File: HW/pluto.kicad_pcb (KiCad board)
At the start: 4 copper layers, 99.8 x 99.8 mm, 68 parts, among them J1 VCC1, J10 GND3, J11 Expansion Bus, J12 VIA2PB, J2 GND1, J3 VCC2, J4 POWER, J5 GND2, J6 RS232a, J9 VCC3, P1 IDE0, Q1 DS1813, SW1 RESET, SW2 PANIC, U1 WD65C02PLCC44, U10 MAX232, U11 ST16C550PLCC44, U12 74LS03, U2 AT28HC256EPLCC32, U3 IS61C256AL-12JLI, U4 DS1511Y+, U5 TL7705B, U6 PlutoDecoder, U7 WD65C22PLCC44, U8 74HC74, U9 WD65C22PLCC44, X1 16MHz, X2 3.6864MHz

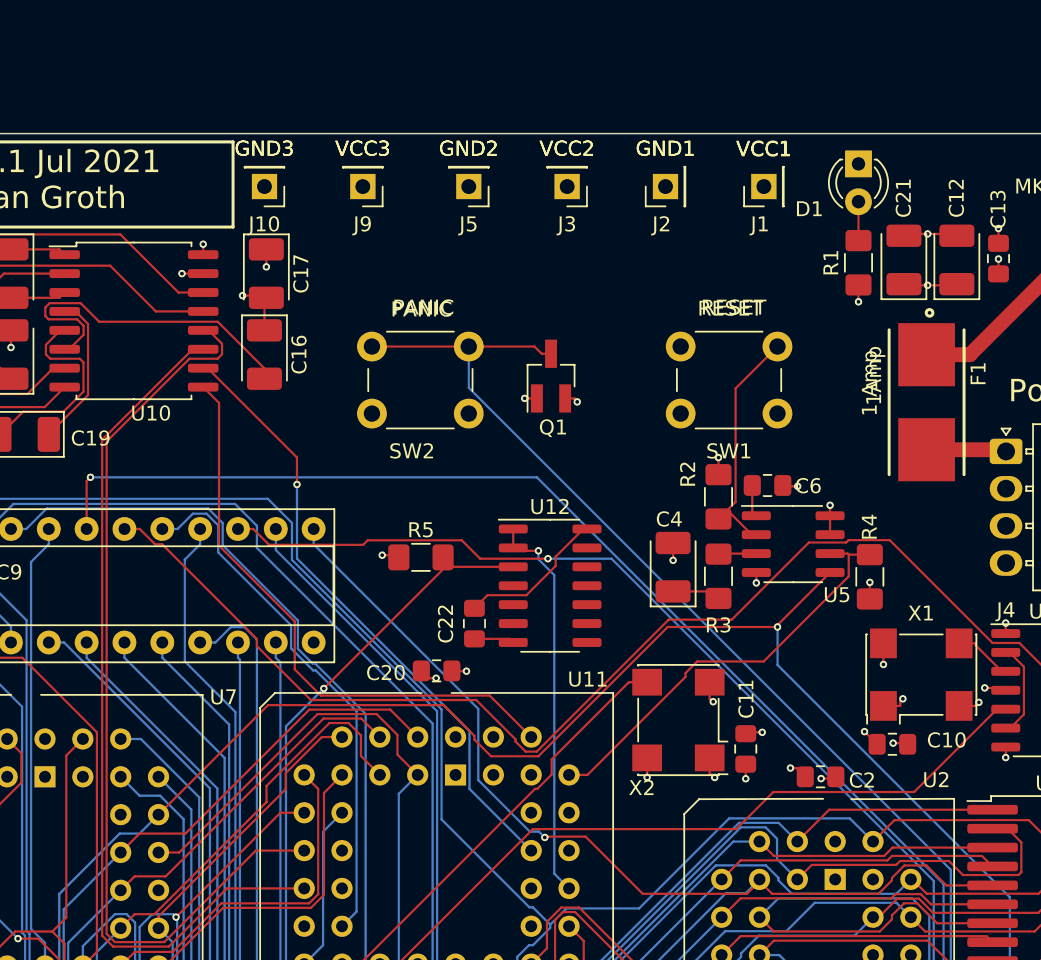
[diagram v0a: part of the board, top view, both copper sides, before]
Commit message: small updates
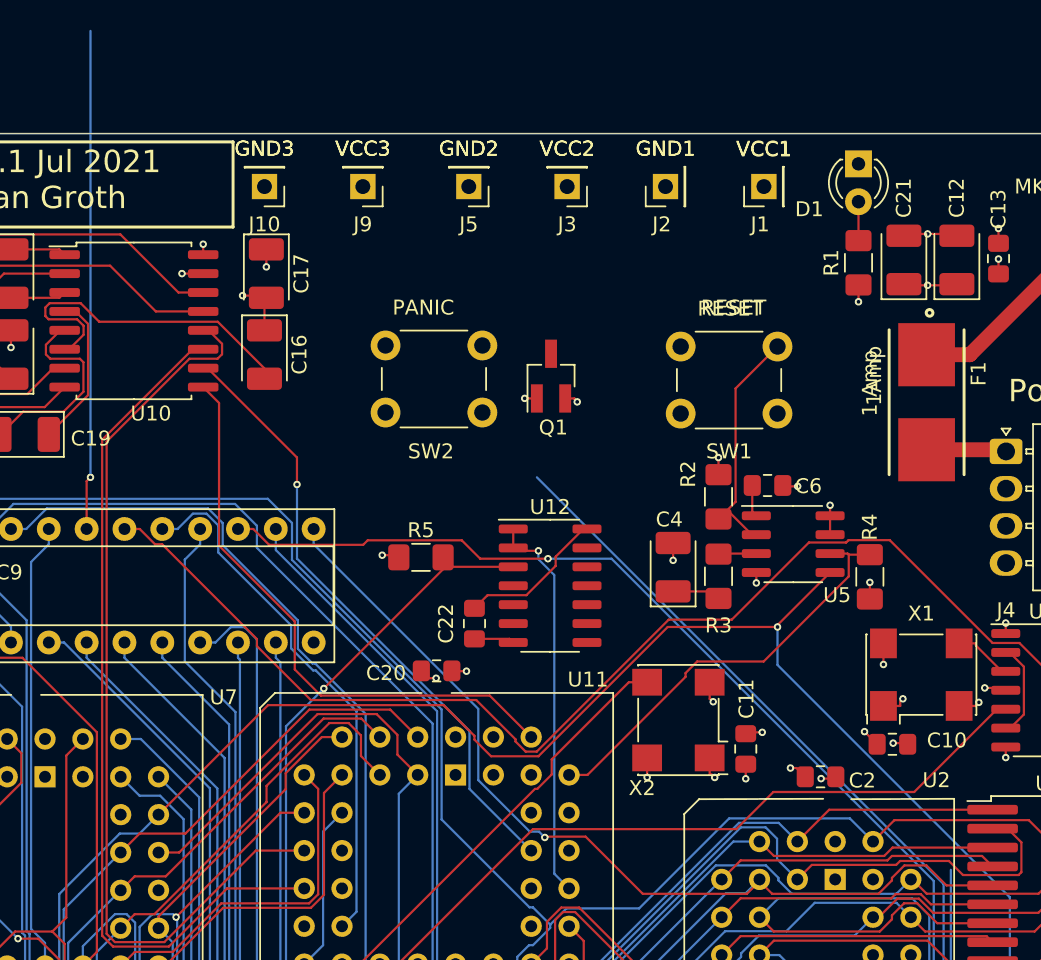
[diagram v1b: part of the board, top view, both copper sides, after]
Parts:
- moved SW2 7.22 mm to (102.0, 54.4), turned to 0 degrees
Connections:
- net Net-(U11-Pad18) renamed /DUART and RS232/UART_CLK
- C22 pad 1: Net-(C22-Pad1) -> GND
- C22 pad 2: Net-(C22-Pad2) -> VCC
- Q1 pad 1: GND -> /Address decoding and support section/~NMI
- Q1 pad 3: /Address decoding and support section/~NMI -> GND
- U12 pad 14: Net-(C22-Pad2) -> VCC
- U12 pad 7: Net-(C22-Pad1) -> GND
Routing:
- net /Address decoding and support section/~NMI: track 147.3 -> 87.3 mm, vias 1 -> 2
- net VCC: track 42.5 -> 52.6 mm
- net Net-(C22-Pad2): track 10.1 -> 0.00 mm
- net Net-(C22-Pad1): track 2.71 -> 0.00 mm
- net GND: track 39.7 -> 41.6 mm, vias 24 -> 23
